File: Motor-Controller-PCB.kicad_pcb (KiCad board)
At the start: 2 copper layers, 26 parts, among them Q1 AO3401A, Q1 TO-252-2

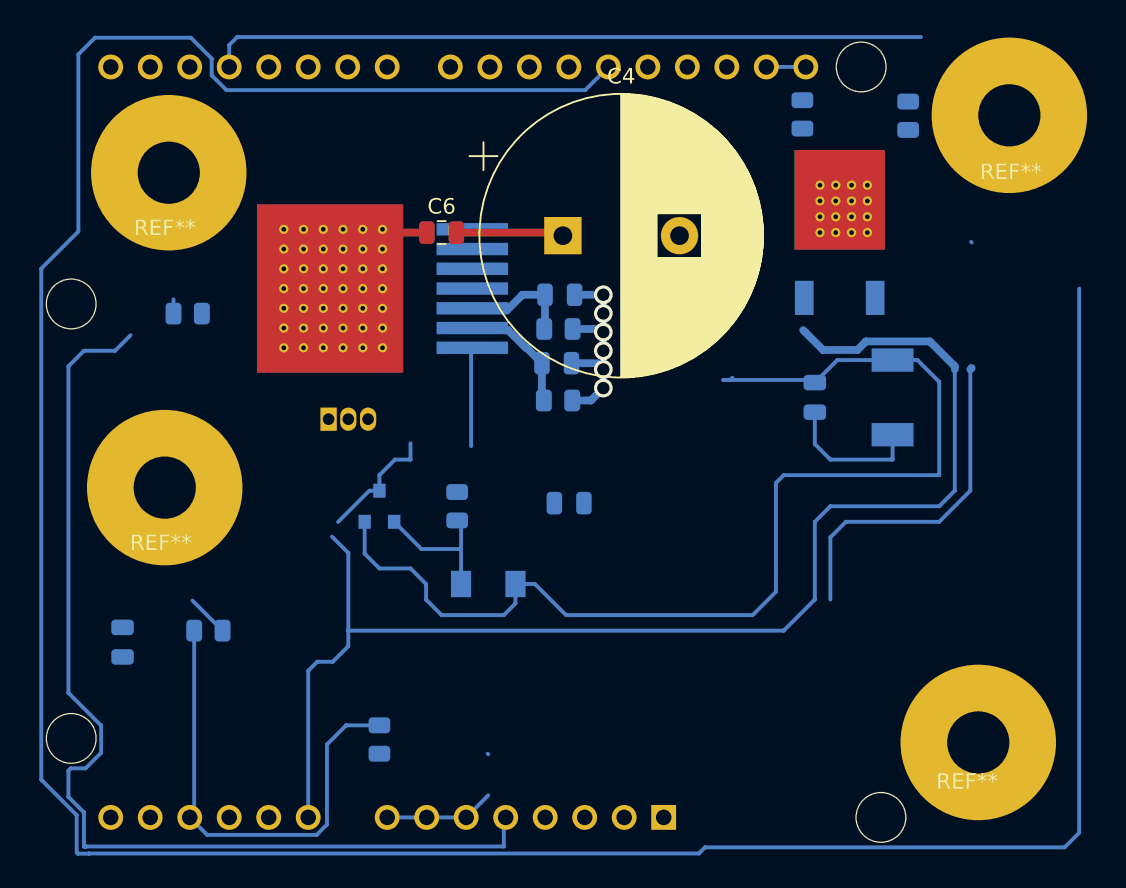
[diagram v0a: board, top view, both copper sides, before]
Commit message: layouting
layouting
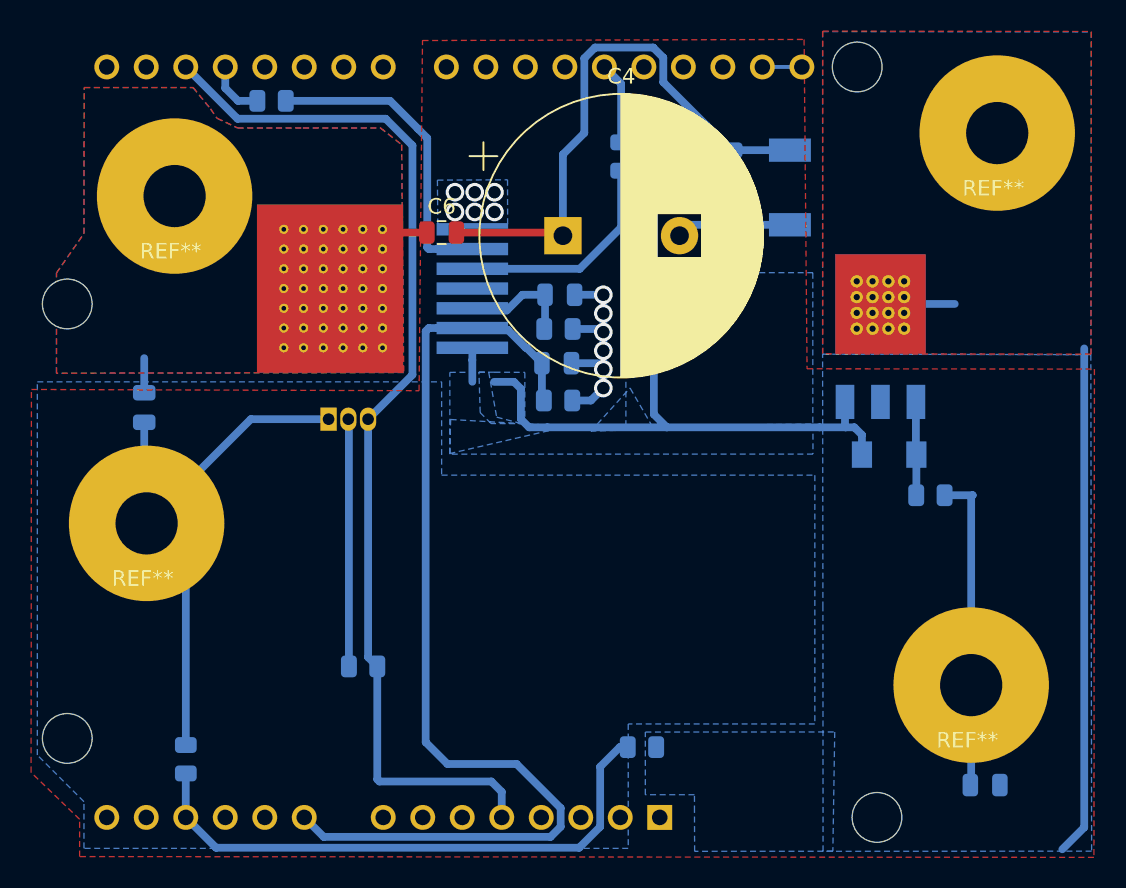
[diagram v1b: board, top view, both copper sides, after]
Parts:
- removed the Q1 at (167.6, 83.4)
- removed the Q1 at (138.0, 101.0)
- removed the REF** at (123.9, 102.8)
- removed the REF** at (178.6, 79.0)
- removed the REF** at (175.8, 118.2)
- removed the REF** at (124.2, 82.6)
- added Q1: IPD90P04P4L, Motor-Controller-PCB:TO-252-3_TabPin2, B.Cu at (170.2, 90.1)
- added REF**: Giant_Green_Circle, Motor-Controller-PCB:Giant_Green_Circle, F.Cu at (122.8, 105.2)
- added REF**: Giant_Green_Circle, Motor-Controller-PCB:Giant_Green_Circle, F.Cu at (175.8, 115.5)
- added REF**: Giant_Green_Circle, Motor-Controller-PCB:Giant_Green_Circle, F.Cu at (177.5, 80.0)
- added REF**: Giant_Green_Circle, Motor-Controller-PCB:Giant_Green_Circle, F.Cu at (124.6, 84.1)
- moved C12 56.2 mm to (176.9, 118.9), turned to 0 degrees
- moved R1 40.9 mm to (131.1, 74.9), turned to 180 degrees
- moved R15 30.4 mm to (173.4, 100.3), turned to 0 degrees
- moved R13 28.9 mm to (154.9, 116.5)
- moved C5 28.0 mm to (122.9, 94.7), turned to 90 degrees
- moved D3 27.1 mm to (170.8, 97.7), turned to 0 degrees
- moved R12 25.3 mm to (136.9, 111.3), turned to 0 degrees
- moved C14 15.9 mm to (160.6, 79.0)
- moved D2 15.0 mm to (164.4, 80.5)
- moved R14 12.5 mm to (125.5, 117.3), turned to 90 degrees
- moved R5 12.0 mm to (153.5, 78.5), turned to 270 degrees
- moved A1 0.25 mm to (184.0, 123.5)
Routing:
- net Net-(A1-Pad27): track 190.5 -> 5.29 mm
- net Net-(A1-Pad18): track 46.1 -> 3.77 mm
- net GNDREF: track 52.4 -> 83.5 mm, vias 6 -> 12
- net VBAT: track 10.7 -> 37.6 mm
- net Net-(A1-Pad9): track 92.7 -> 68.4 mm
- net Net-(DEV.1-Pad2): track 0.00 -> 22.3 mm
- net Net-(R12-Pad1): track 0.00 -> 15.9 mm
- net Net-(DEV.1-Pad3): track 0.00 -> 14.3 mm
- net Net-(A1-Pad12): track 30.7 -> 37.4 mm
- net Net-(C14-Pad1): track 86.3 -> 89.6 mm
- net Net-(D3-Pad2): track 9.22 -> 6.03 mm
- net OUT_1: track 8.29 -> 10.5 mm
- net 5V_ARDUINO: track 68.3 -> 69.0 mm
- added copper zone on B.Cu, net GNDREF
- added copper zone on F.Cu, net GNDREF
- added copper zone on B.Cu, net Net-(C14-Pad1)
- added copper zone on B.Cu, net OUT_1
- added copper zone on F.Cu, net OUT_1
- added copper zone on B.Cu, net VBAT
- added copper zone on F.Cu, net VBAT
